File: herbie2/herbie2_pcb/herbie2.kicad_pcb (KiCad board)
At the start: 2 copper layers, 120.7 x 97.8 mm, 42 parts, among them J1 GND, J10 CONN_04JST-PTH, J11 CONN_04JST-PTH, J2 5V, J3 I2C_STANDARDQWIIC, J4 Servo0, J5 Servo1, J6 Servo2, J7 Servo3, J8 I2C_STANDARDQWIIC, J9 I2C_STANDARDQWIIC, Q1 LTC4412, Q2 LTC4412, Q3 Si4427, Q4 Si4427, U1 74164, U1 74HC595, U2 74164, U3 24v13_Pololu, U4 LS7366R, U5 LS7366R, U6 TCA9534, U7 24v13_Pololu

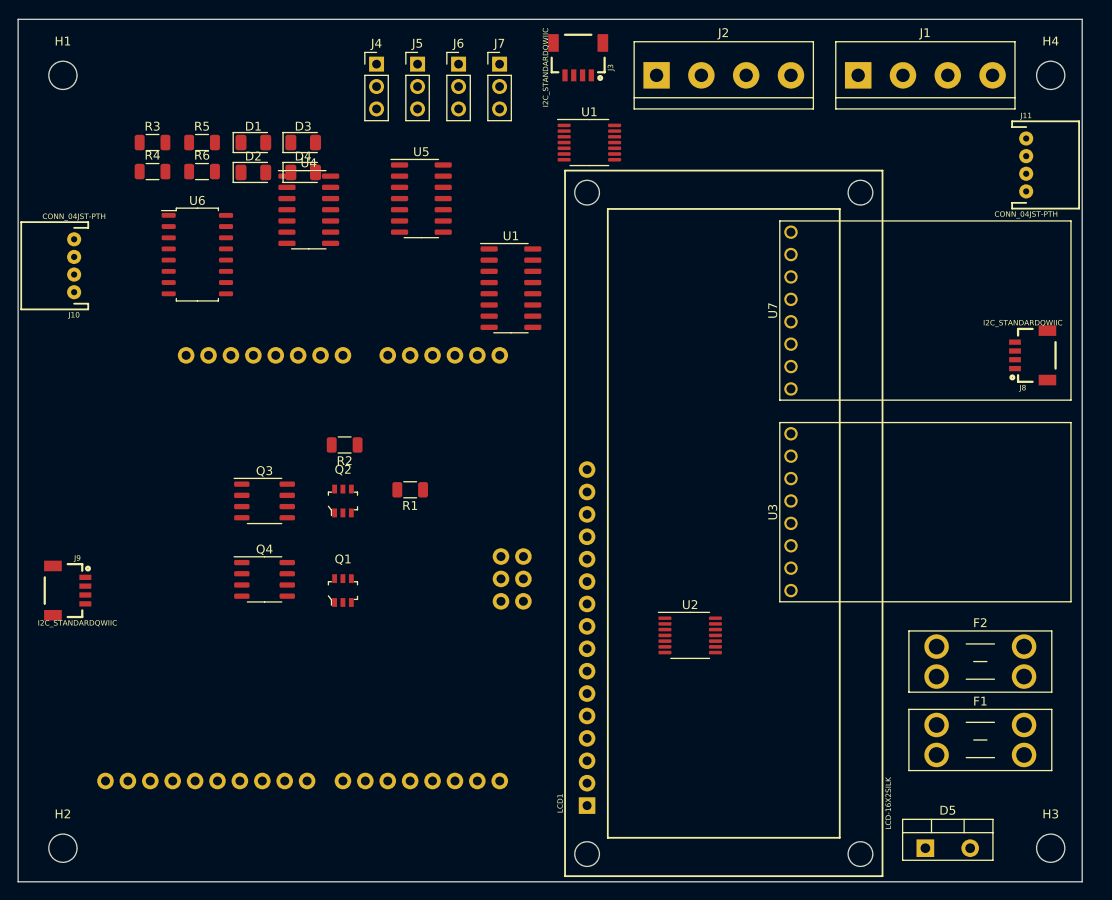
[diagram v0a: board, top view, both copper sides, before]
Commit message: updated PCB
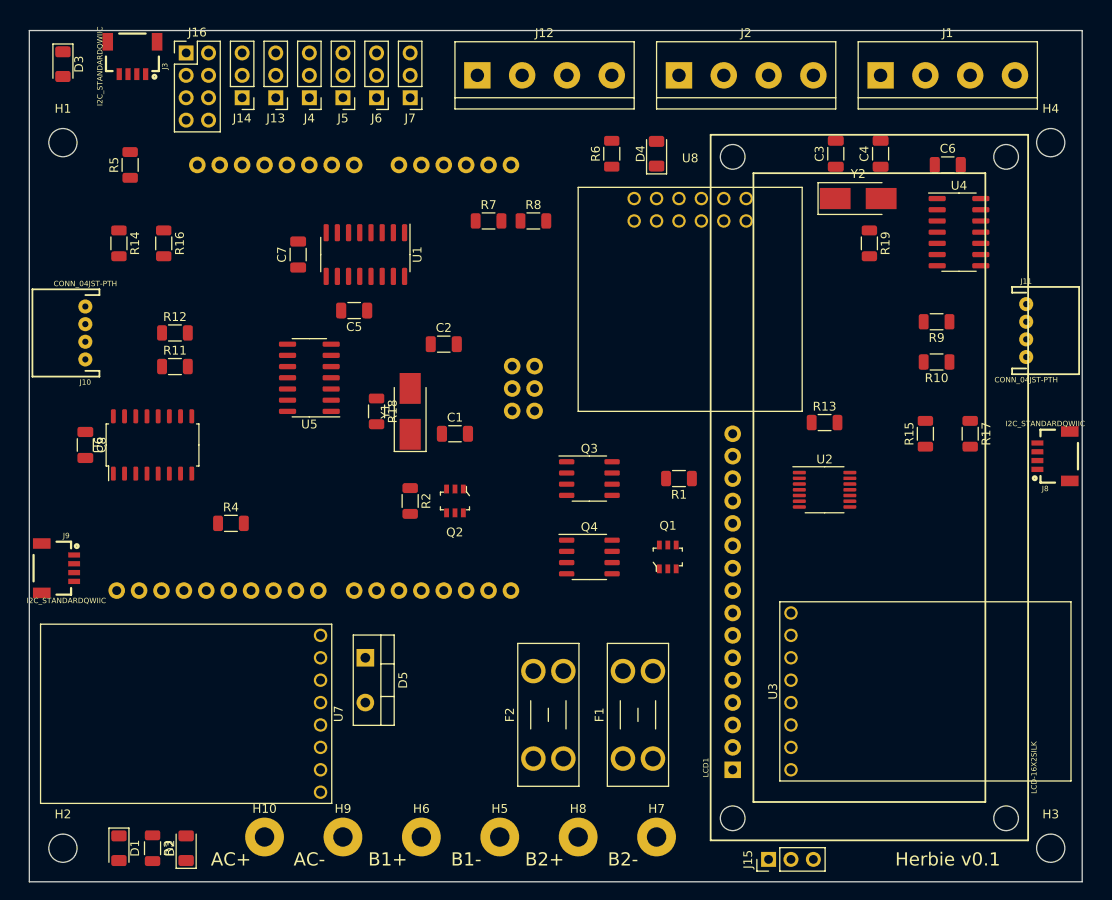
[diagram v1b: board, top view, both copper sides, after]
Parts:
- removed the U1 at (166.4, 52.1)
- added C1: 12pF, Capacitor_SMD:C_1206_3216Metric, F.Cu at (151.1, 85.1)
- added C2: 12pF, Capacitor_SMD:C_1206_3216Metric, F.Cu at (149.9, 74.9)
- added C3: 12pF, Capacitor_SMD:C_1206_3216Metric, F.Cu at (194.3, 53.3)
- added C4: 12pF, Capacitor_SMD:C_1206_3216Metric, F.Cu at (199.4, 53.3)
- added C5: .1uF, Capacitor_SMD:C_1206_3216Metric, F.Cu at (139.7, 71.1)
- added C6: .1uF, Capacitor_SMD:C_1206_3216Metric, F.Cu at (207.0, 54.6)
- added C7: .1uF, Capacitor_SMD:C_1206_3216Metric, F.Cu at (133.3, 64.8)
- added C8: .1uF, Capacitor_SMD:C_1206_3216Metric, F.Cu at (109.2, 86.4)
- added H10: AC_PWR, MountingHole:MountingHole_2.2mm_M2_Pad, F.Cu at (129.5, 130.8)
- added H5: GND_BATT1, MountingHole:MountingHole_2.2mm_M2_Pad, F.Cu at (156.2, 130.8)
- added H6: PWR_BATT1, MountingHole:MountingHole_2.2mm_M2_Pad, F.Cu at (147.3, 130.8)
- added H7: GND_BATT2, MountingHole:MountingHole_2.2mm_M2_Pad, F.Cu at (174.0, 130.8)
- added H8: PWR_BATT2, MountingHole:MountingHole_2.2mm_M2_Pad, F.Cu at (165.1, 130.8)
- added H9: GND_AC_PWR, MountingHole:MountingHole_2.2mm_M2_Pad, F.Cu at (138.4, 130.8)
- added J12: Vin, TerminalBlock:TerminalBlock_bornier-4_P5.08mm, F.Cu at (153.7, 44.5)
- added J13: Servo4, Connector_PinHeader_2.54mm:PinHeader_1x03_P2.54mm_Vertical, F.Cu at (130.8, 47.0)
- added J14: Servo5, Connector_PinHeader_2.54mm:PinHeader_1x03_P2.54mm_Vertical, F.Cu at (127.0, 47.0)
- added J15: Conn_01x03_Male, Connector_PinHeader_2.54mm:PinHeader_1x03_P2.54mm_Vertical, F.Cu at (186.7, 133.3)
- added J16: Conn_02x04_Odd_Even, Connector_PinHeader_2.54mm:PinHeader_2x04_P2.54mm_Vertical, F.Cu at (120.7, 41.9)
- added R10: 100, Resistor_SMD:R_1206_3216Metric, F.Cu at (205.7, 77.0)
- added R11: 100, Resistor_SMD:R_1206_3216Metric, F.Cu at (119.4, 77.5)
- added R12: 100, Resistor_SMD:R_1206_3216Metric, F.Cu at (119.4, 73.7)
- added R13: 10, Resistor_SMD:R_1206_3216Metric, F.Cu at (193.0, 83.8)
- added R14: 20K, Resistor_SMD:R_1206_3216Metric, F.Cu at (113.0, 63.5)
- added R15: 20K, Resistor_SMD:R_1206_3216Metric, F.Cu at (204.5, 85.1)
- added R16: 20K, Resistor_SMD:R_1206_3216Metric, F.Cu at (118.1, 63.5)
- added R17: 20K, Resistor_SMD:R_1206_3216Metric, F.Cu at (209.6, 85.1)
- added R18: 1M, Resistor_SMD:R_1206_3216Metric, F.Cu at (142.2, 82.5)
- added R19: 1M, Resistor_SMD:R_1206_3216Metric, F.Cu at (198.1, 63.5)
- added R7: R, Resistor_SMD:R_1206_3216Metric, F.Cu at (154.9, 61.0)
- added R8: R, Resistor_SMD:R_1206_3216Metric, F.Cu at (160.0, 61.0)
- added R9: 100, Resistor_SMD:R_1206_3216Metric, F.Cu at (205.7, 72.4)
- added U8: D36V50F5_Pololu, js:D36V50F5_Pololu, F.Cu at (177.8, 69.8)
- added Y1: 20MHz, Crystal:Crystal_SMD_5032-2Pin_5.0x3.2mm_HandSoldering, F.Cu at (146.1, 82.5)
- added Y2: 20MHz, Crystal:Crystal_SMD_5032-2Pin_5.0x3.2mm_HandSoldering, F.Cu at (196.8, 58.4)
- J4: value Servo0 -> Servo3
- J5: value Servo1 -> Servo2
- J6: value Servo2 -> Servo1
- J7: value Servo3 -> Servo0
- moved U7 93.3 mm to (121.9, 116.8), turned to 270 degrees
- moved D1 81.4 mm to (113.0, 132.1), turned to 270 degrees
- moved R3 80.0 mm to (116.8, 132.1), turned to 270 degrees
- moved D2 77.0 mm to (120.7, 132.1), turned to 90 degrees
- moved U4 73.8 mm to (208.3, 62.2)
- moved D5 67.1 mm to (141.0, 110.5), turned to 270 degrees
- moved J3 50.5 mm to (114.6, 44.3)
- moved F2 47.5 mm to (160.0, 121.9), turned to 90 degrees
- moved R6 46.5 mm to (168.9, 53.3), turned to 90 degrees
- moved R4 40.9 mm to (125.7, 95.2)
- moved D4 40.1 mm to (174.0, 53.3), turned to 90 degrees
- moved Q1 37.0 mm to (175.3, 99.1)
- moved Q3 36.9 mm to (166.4, 90.2)
- moved Q4 36.9 mm to (166.4, 99.1)
- moved F1 35.8 mm to (170.2, 121.9), turned to 90 degrees
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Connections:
- B2 pad 5V: 5V -> 5V_USB
- J1 pad 1: Net-(J1-Pad1) -> GND
- J1 pad 2: Net-(J1-Pad2) -> GND
- J1 pad 3: Net-(J1-Pad3) -> GND
- J1 pad 4: Net-(J1-Pad4) -> GND
- J2 pad 1: Net-(J2-Pad1) -> 5V
- J2 pad 2: Net-(J2-Pad2) -> 5V
- J2 pad 3: Net-(J2-Pad3) -> 5V
- J2 pad 4: Net-(J2-Pad4) -> 5V
- LCD1 pad 16: Net-(LCD1-Pad16) -> GND
- U3 pad 4: Net-(U3-Pad4) -> E_STOP1
- U4 pad 11: Net-(J11-Pad4) -> Net-(R10-Pad2)
- U4 pad 12: Net-(J11-Pad3) -> Net-(R9-Pad2)
- U5 pad 11: Net-(J10-Pad4) -> Net-(R12-Pad2)
- U5 pad 12: Net-(J10-Pad3) -> Net-(R11-Pad2)
- U6 pad 10: Net-(U6-Pad10) -> DI1
- U6 pad 11: Net-(U6-Pad11) -> DI2
- U6 pad 12: Net-(U6-Pad12) -> DI3
- U6 pad 9: Net-(U6-Pad9) -> DI0
- U7 pad 4: Net-(U7-Pad4) -> E_STOP2
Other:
- board size 120.7 x 97.8 mm -> 119.4 x 96.5 mm
- board text added: "AC+"
- board text added: "AC-"
- board text added: "B1+"
- board text added: "B1-"
- board text added: "B2+"
- board text added: "B2-"
- board text added: "Herbie v0.1"
